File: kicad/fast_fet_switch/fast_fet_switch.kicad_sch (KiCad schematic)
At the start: 20 parts, among them J1 Conn_01x03_Pin, J2 Conn_01x03_Pin, J3 Conn_01x09_Pin, J4 Conn_01x01_Pin, J5 Conn_01x01_Pin, Q1 IRF4905, Q2 IRF4905, Q3 BS170, U1 TXS0108EPW, U2 AP2127K-1.8, U4 XIAO-RP2040-SMD, U5 AP2112K-1.2

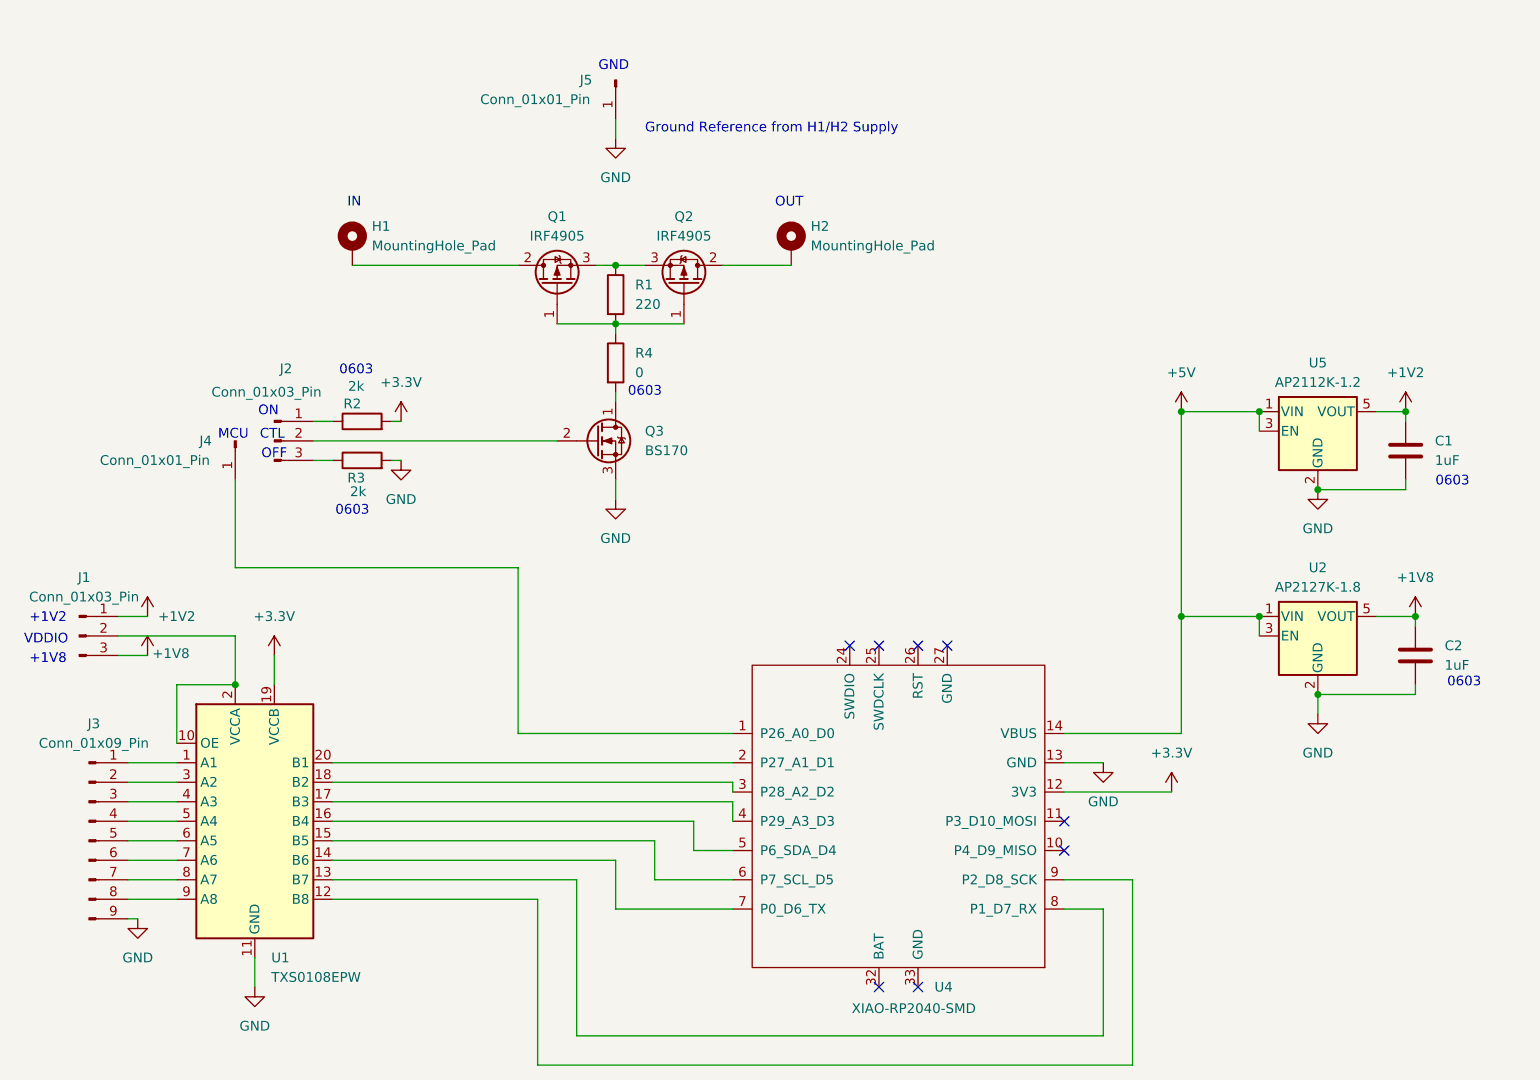
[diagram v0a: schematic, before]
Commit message: Add files via upload
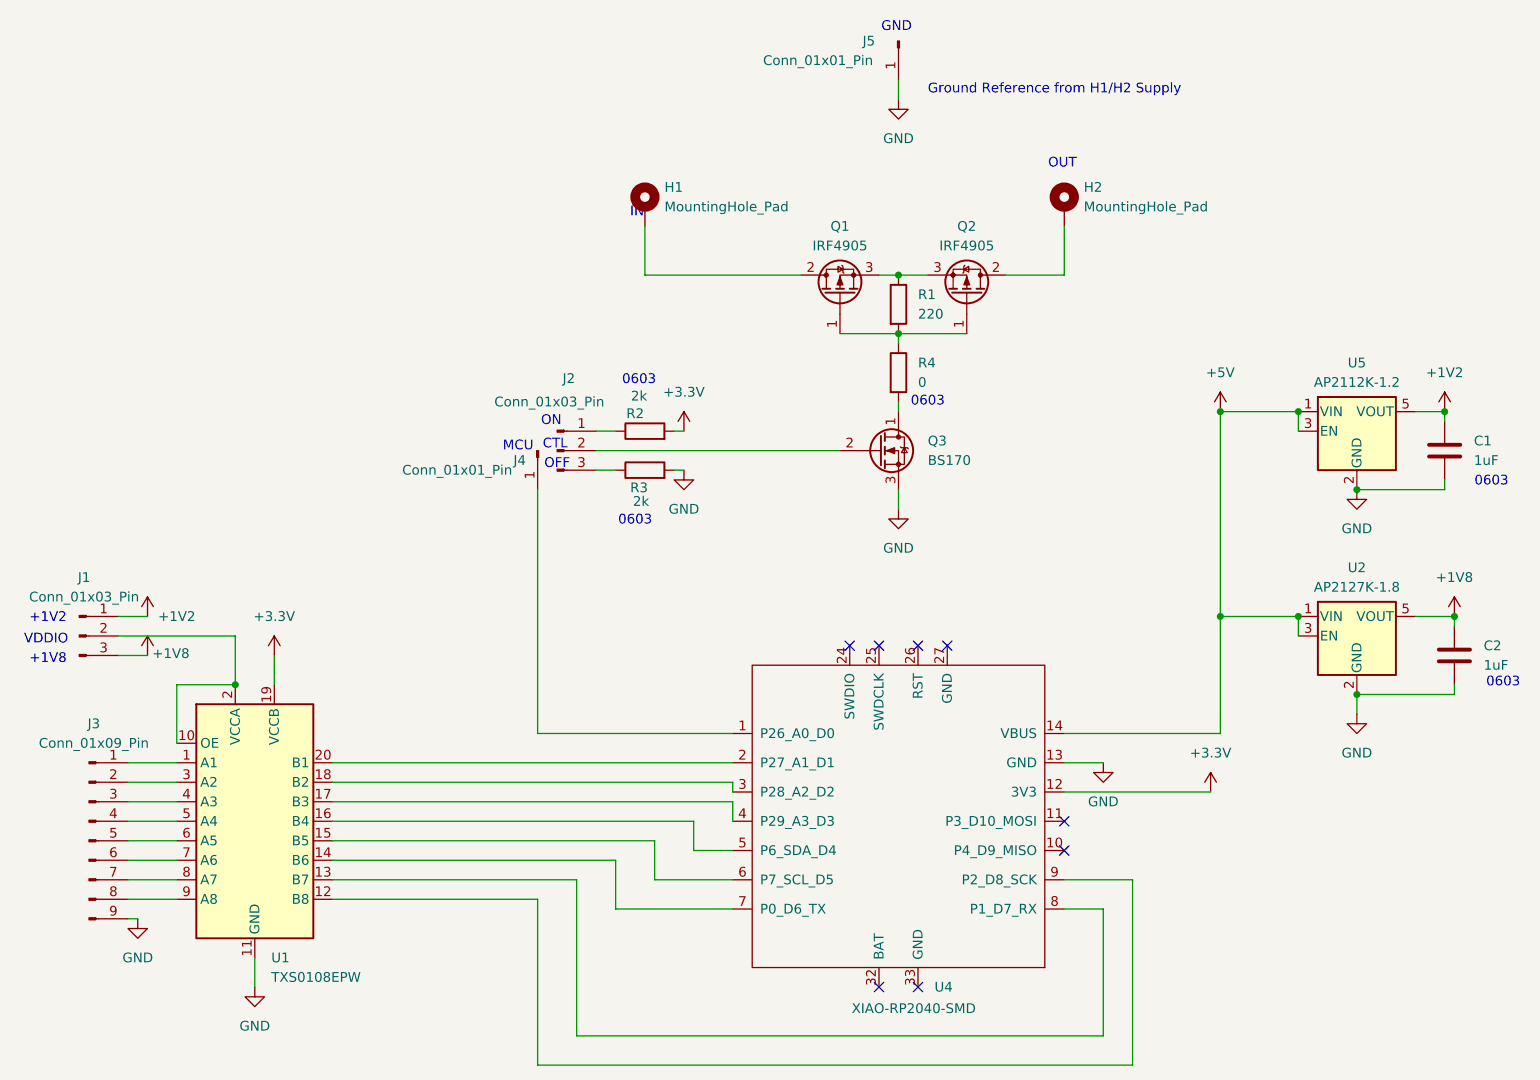
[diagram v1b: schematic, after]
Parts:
- R1, R2, R3, R4: footprint Resistor_SMD:R_0201_0603Metric -> Resistor_SMD:R_0603_1608Metric
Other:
- moved on the sheet: C1, C2, H1, H2, J2, J4, J5, Q1, Q2, Q3, R1, R2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

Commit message: Add files via upload
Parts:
- C1, C2: footprint Capacitor_SMD:C_0201_0603Metric -> Capacitor_SMD:C_0603_1608Metric
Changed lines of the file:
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@@
 			)
 		)
-		(property "Footprint" "Capacitor_SMD:C_0201_0603Metric"
+		(property "Footprint" "Capacitor_SMD:C_0603_1608Metric"
 			(at 225.7552 78.74 0)
 			(hide yes)
@@
 			)
 		)
-		(property "Footprint" "Capacitor_SMD:C_0201_0603Metric"
+		(property "Footprint" "Capacitor_SMD:C_0603_1608Metric"
 			(at 227.0252 105.41 0)
 			(hide yes)
